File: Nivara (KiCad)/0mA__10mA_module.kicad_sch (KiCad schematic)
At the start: 4 parts, among them U7 GP8201S-TC50-EW

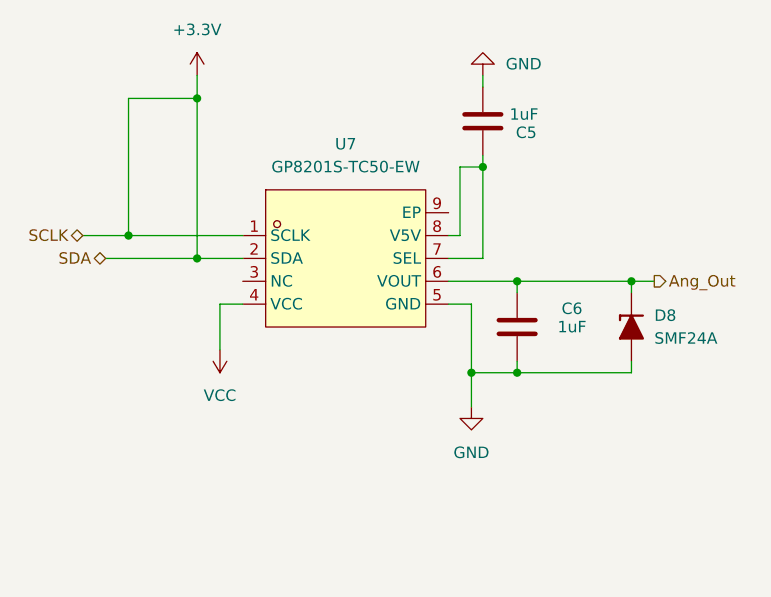
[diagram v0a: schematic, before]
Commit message: Add files via upload
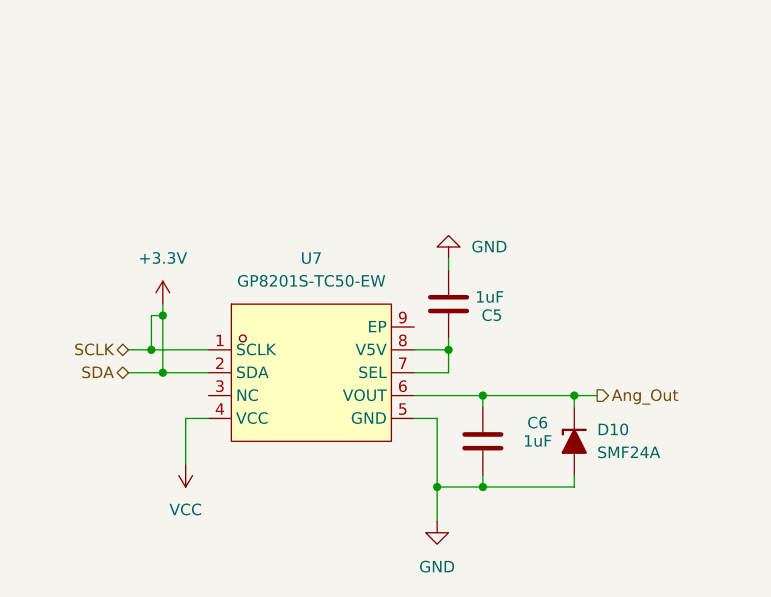
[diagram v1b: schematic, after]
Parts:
- C5, C6: footprint PCM_Capacitor_SMD_AKL:C_0603_1608Metric -> Capacitor_SMD:C_0402_1005Metric
- D10: renamed from D8; footprint PCM_Diode_SMD_AKL:D_SOD-123F -> Diode_SMD:D_SMF
- U7: footprint EastEDA:GP8303-TC50-EW -> External:GP8201S
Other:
- moved on the sheet: C5, C6, D10, U7
